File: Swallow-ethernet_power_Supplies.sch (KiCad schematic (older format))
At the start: 31 parts, among them P7 +5V_In, P8 V_In, U12 NCP1529, U13 NCP1529, U14 NCP303LSN09T1G

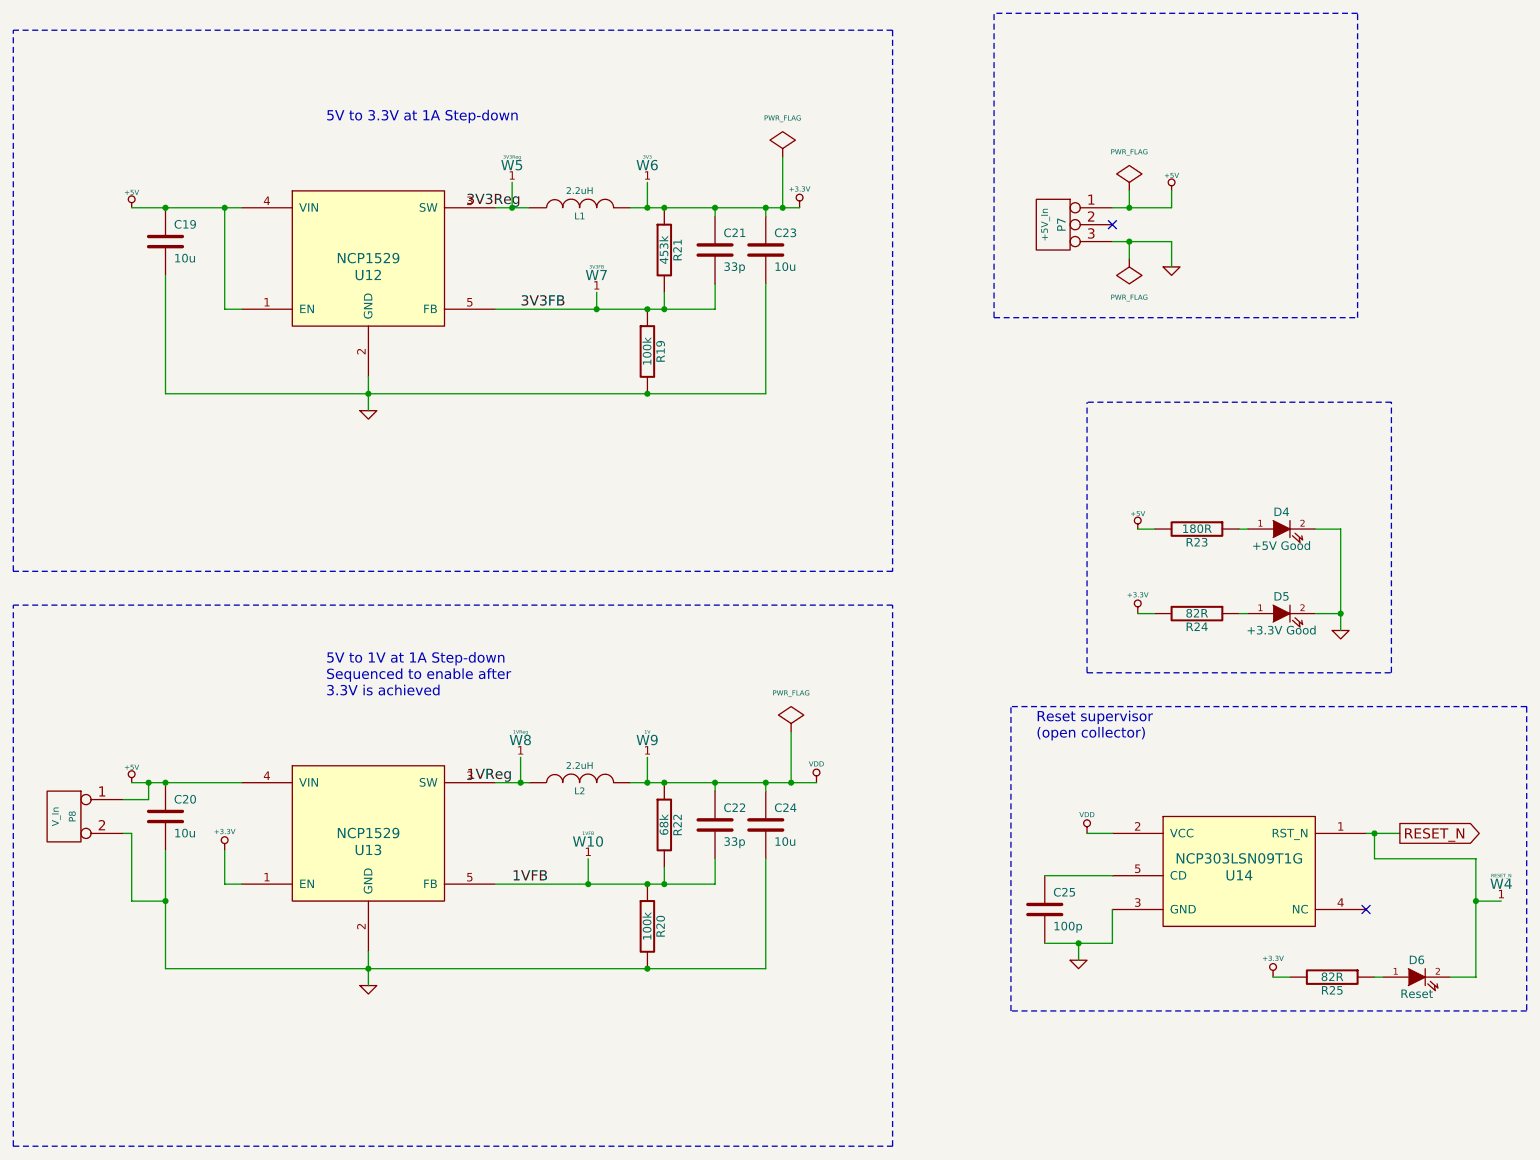
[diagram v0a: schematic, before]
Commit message: Completed schematic.
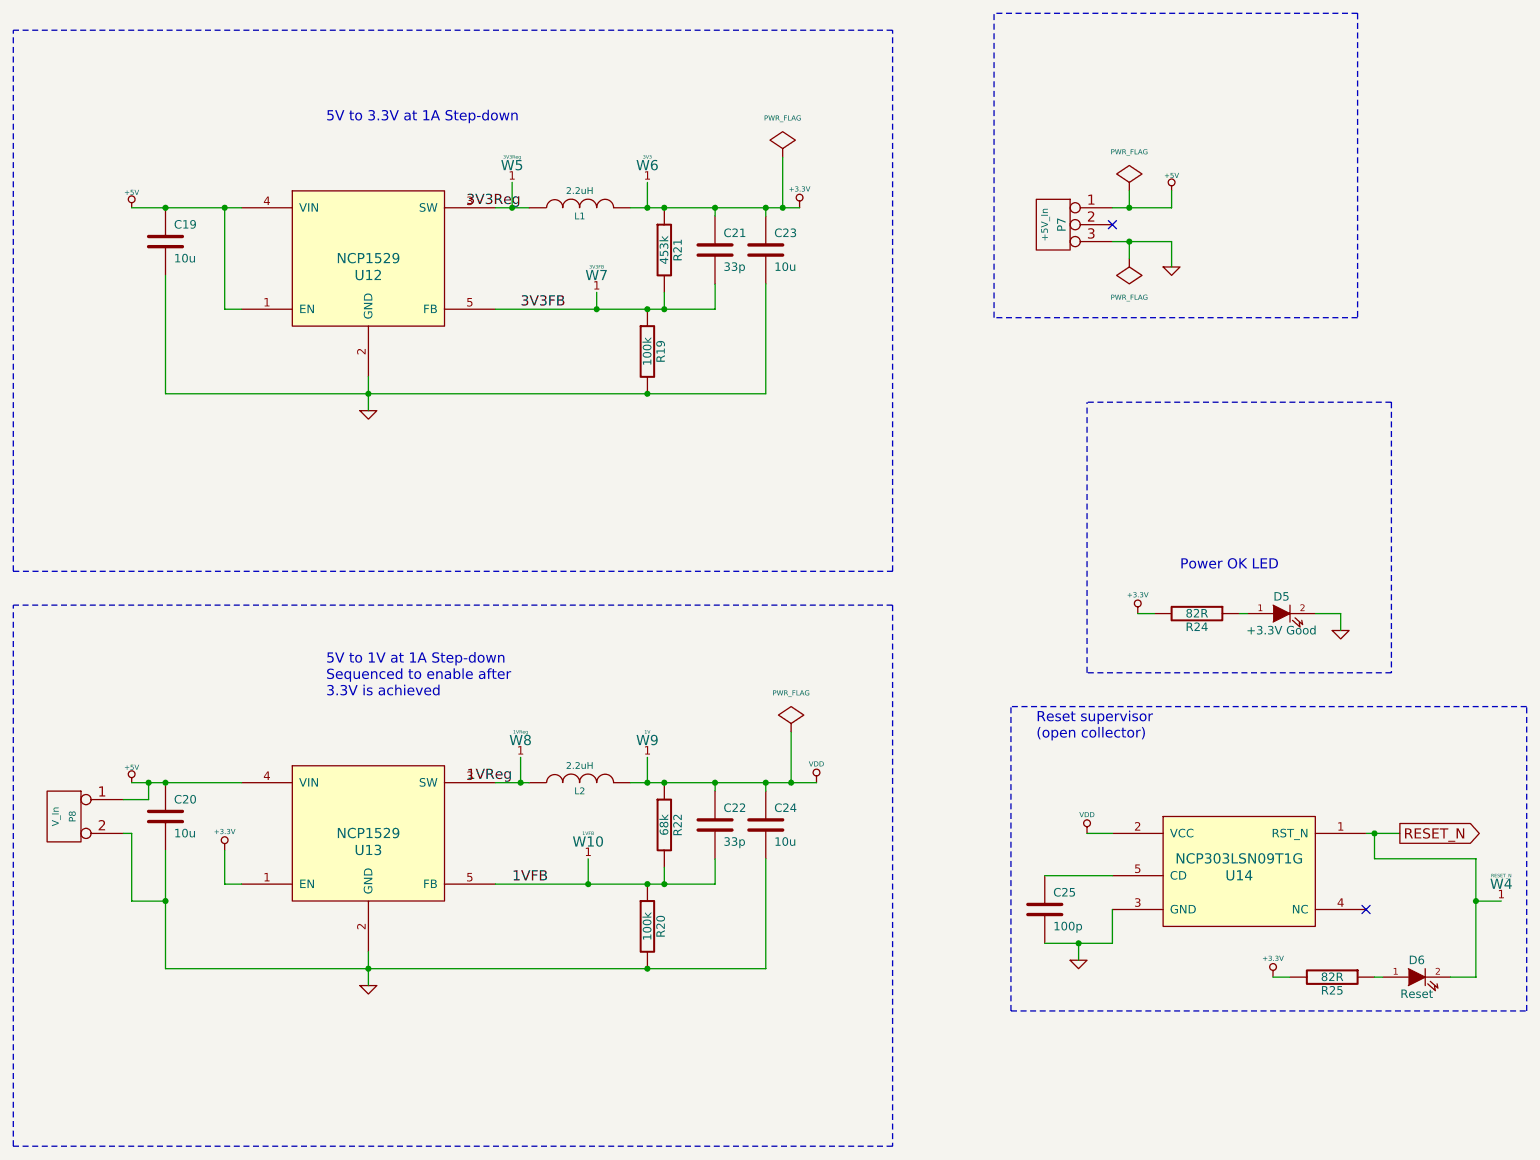
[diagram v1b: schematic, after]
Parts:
- removed D4: +5V Good, X_LED-0603, symbol LED
- removed R23: 180R, SM0402, symbol R
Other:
- note added: "Power OK LED"
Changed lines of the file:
@@
-EESchema Schematic File Version 2  date 30/09/2012 20:10:31
+EESchema Schematic File Version 2  date 30/09/2012 22:11:50
 LIBS:power
 LIBS:device
@@
 Comment4 ""
 $EndDescr
-Wire Wire Line
-	7550 2200 7900 2200
+Text Notes 7950 4150 0    60   ~ 0
+Power OK LED
+Wire Wire Line
+	8900 4500 8900 4400
+Wire Wire Line
+	7650 2200 7650 2300
+Wire Wire Line
+	1700 5700 1750 5700
+Wire Wire Line
+	1750 5700 1750 6100
+Connection ~ 1950 6100
+Wire Wire Line
+	1750 6100 1950 6100
+Connection ~ 4800 5400
+Wire Wire Line
+	4800 5250 4800 5400
+Connection ~ 4000 2000
+Wire Wire Line
+	4000 1850 4000 2000
+Connection ~ 4500 2600
+Wire Wire Line
+	4500 2500 4500 2600
+Connection ~ 9100 5700
+Wire Wire Line
+	9100 5700 9100 5850
+Wire Wire Line
+	9100 5850 9700 5850
+Wire Wire Line
+	9700 5850 9700 6550
+Wire Notes Line
+	6950 6750 6950 4950
+Wire Notes Line
+	6950 6750 10000 6750
+Wire Notes Line
+	10000 6750 10000 4950
+Wire Notes Line
+	10000 4950 6950 4950
+Wire Wire Line
+	9050 5700 9250 5700
+Connection ~ 7350 6350
+Wire Wire Line
+	7350 6450 7350 6350
+Wire Wire Line
+	7150 6350 7550 6350
+Wire Wire Line
+	7550 6350 7550 6150
+Wire Wire Line
+	2400 6000 2300 6000
+Wire Notes Line
+	9200 3150 7400 3150
+Wire Notes Line
+	9200 3150 9200 4750
+Wire Notes Line
+	9200 4750 7400 4750
+Wire Notes Line
+	7400 4750 7400 3150
+Wire Wire Line
+	7700 4400 7800 4400
+Connection ~ 5650 5400
+Wire Wire Line
+	5650 5100 5650 5400
+Wire Wire Line
+	7650 2000 7650 1900
+Connection ~ 7650 2000
+Wire Wire Line
+	7900 2350 7900 2200
+Wire Wire Line
+	5800 5400 4700 5400
+Connection ~ 1950 2000
+Wire Wire Line
+	1750 2000 2400 2000
+Connection ~ 4800 3100
+Wire Wire Line
+	5500 2450 5500 3100
+Wire Wire Line
+	5500 3100 1950 3100
+Connection ~ 4900 2600
+Wire Wire Line
+	3900 2600 5200 2600
+Wire Wire Line
+	5200 2600 5200 2450
+Connection ~ 4900 2000
+Wire Wire Line
+	5200 2000 5200 2050
+Wire Wire Line
+	3900 2000 4100 2000
+Connection ~ 3150 3100
+Wire Wire Line
+	1950 3100 1950 2400
+Wire Wire Line
+	3150 3200 3150 3000
+Wire Wire Line
+	2400 2600 2300 2600
+Wire Wire Line
+	2300 2600 2300 2000
+Connection ~ 2300 2000
+Wire Wire Line
+	4900 2600 4900 2500
+Connection ~ 4800 2600
+Wire Wire Line
+	5500 2050 5500 2000
+Connection ~ 5200 2000
+Wire Wire Line
+	5700 2000 4700 2000
+Connection ~ 5500 2000
+Wire Notes Line
+	1050 4150 1050 950
+Wire Notes Line
+	1050 4150 6250 4150
+Wire Notes Line
+	6250 4150 6250 950
+Wire Notes Line
+	6250 950  1050 950
+Wire Notes Line
+	6250 4350 1050 4350
+Wire Notes Line
+	6250 4350 6250 7550
+Wire Notes Line
+	6250 7550 1050 7550
+Wire Notes Line
+	1050 7550 1050 4350
+Connection ~ 5500 5400
+Connection ~ 5200 5400
+Wire Wire Line
+	5500 5400 5500 5450
+Connection ~ 4800 6000
+Wire Wire Line
+	4900 5900 4900 6000
+Wire Wire Line
+	3150 6600 3150 6400
+Wire Wire Line
+	1950 5800 1950 6500
+Connection ~ 3150 6500
+Wire Wire Line
+	3900 5400 4100 5400
+Wire Wire Line
+	5200 5400 5200 5450
+Connection ~ 4900 5400
+Wire Wire Line
+	5200 5850 5200 6000
+Wire Wire Line
+	5200 6000 3900 6000
+Connection ~ 4900 6000
+Wire Wire Line
+	1950 6500 5500 6500
+Wire Wire Line
+	5500 6500 5500 5850
+Connection ~ 4800 6500
+Wire Wire Line
+	1750 5400 2400 5400
+Connection ~ 1950 5400
+Wire Wire Line
+	7900 1900 7900 2000
+Wire Notes Line
+	9000 850  6850 850
+Wire Notes Line
+	9000 850  9000 2650
+Wire Notes Line
+	9000 2650 6850 2650
+Wire Notes Line
+	6850 2650 6850 850
+Connection ~ 7650 2200
+Wire Wire Line
+	5600 1700 5600 2000
+Connection ~ 5600 2000
+Wire Wire Line
+	8900 4400 8750 4400
+Wire Wire Line
+	8300 4400 8350 4400
+Wire Wire Line
+	7550 5950 7150 5950
+Wire Wire Line
+	7400 5700 7550 5700
+Wire Wire Line
+	9100 6550 9150 6550
+Wire Wire Line
+	9700 6550 9550 6550
+Wire Wire Line
+	8500 6550 8600 6550
+Wire Wire Line
+	9850 6100 9700 6100
+Connection ~ 9700 6100
+Wire Wire Line
+	7900 2000 7550 2000
+Wire Wire Line
+	2300 6000 2300 5800
+Wire Wire Line
+	4800 1850 4800 2000
+Connection ~ 4800 2000
+Wire Wire Line
+	4450 5850 4450 6000
+Connection ~ 4450 6000
+Wire Wire Line
+	4050 5250 4050 5400
+Connection ~ 4050 5400
+Wire Wire Line
+	1700 5500 1850 5500
+Wire Wire Line
+	1850 5500 1850 5400
 Connection ~ 1850 5400
 Wire Wire Line
-	1850 5400 1850 5500
-Wire Wire Line
-	1850 5500 1700 5500
-Connection ~ 4050 5400
-Wire Wire Line
-	4050 5250 4050 5400
-Connection ~ 4450 6000
-Wire Wire Line
-	4450 5850 4450 6000
-Connection ~ 4800 2000
-Wire Wire Line
-	4800 1850 4800 2000
-Wire Wire Line
-	2300 5800 2300 6000
-Wire Wire Line
-	7550 2000 7900 2000
-Connection ~ 9700 6100
-Wire Wire Line
-	9850 6100 9700 6100
-Wire Wire Line
-	8500 6550 8600 6550
-Wire Wire Line
-	9550 6550 9700 6550
-Wire Wire Line
-	9100 6550 9150 6550
-Wire Wire Line
-	7400 5700 7550 5700
-Wire Wire Line
-	7550 5950 7150 5950
-Wire Wire Line
-	8300 4400 8350 4400
-Wire Wire Line
-	7700 3900 7800 3900
-Wire Wire Line
-	8900 4400 8750 4400
-Connection ~ 5600 2000
-Wire Wire Line
-	5600 1700 5600 2000
-Connection ~ 7650 2200
-Wire Notes Line
-	6850 2650 6850 850
-Wire Notes Line
-	6850 2650 9000 2650
-Wire Notes Line
-	9000 2650 9000 850
-Wire Notes Line
-	9000 850  6850 850
-Wire Wire Line
-	7900 2000 7900 1900
-Connection ~ 1950 5400
-Wire Wire Line
-	1750 5400 2400 5400
-Connection ~ 4800 6500
-Wire Wire Line
-	5500 5850 5500 6500
-Wire Wire Line
-	5500 6500 1950 6500
-Connection ~ 4900 6000
-Wire Wire Line
-	3900 6000 5200 6000
-Wire Wire Line
-	5200 6000 5200 5850
-Connection ~ 4900 5400
-Wire Wire Line
-	5200 5400 5200 5450
-Wire Wire Line
-	3900 5400 4100 5400
-Connection ~ 3150 6500
-Wire Wire Line
-	1950 6500 1950 5800
-Wire Wire Line
-	3150 6600 3150 6400
-Wire Wire Line
-	4900 5900 4900 6000
-Connection ~ 4800 6000
-Wire Wire Line
-	5500 5400 5500 5450
-Connection ~ 5200 5400
-Connection ~ 5500 5400
-Wire Notes Line
-	1050 7550 1050 4350
-Wire Notes Line
-	1050 7550 6250 7550
-Wire Notes Line
-	6250 7550 6250 4350
-Wire Notes Line
-	6250 4350 1050 4350
-Wire Notes Line
-	6250 950  1050 950
-Wire Notes Line
-	6250 950  6250 4150
-Wire Notes Line
-	6250 4150 1050 4150
-Wire Notes Line
-	1050 4150 1050 950
-Connection ~ 5500 2000
-Wire Wire Line
-	5700 2000 4700 2000
-Connection ~ 5200 2000
-Wire Wire Line
-	5500 2050 5500 2000
-Connection ~ 4800 2600
-Wire Wire Line
-	4900 2600 4900 2500
-Connection ~ 2300 2000
-Wire Wire Line
-	2300 2000 2300 2600
-Wire Wire Line
-	2300 2600 2400 2600
-Wire Wire Line
-	3150 3200 3150 3000
-Wire Wire Line
-	1950 2400 1950 3100
-Connection ~ 3150 3100
-Wire Wire Line
-	3900 2000 4100 2000
-Wire Wire Line
-	5200 2000 5200 2050
-Connection ~ 4900 2000
-Wire Wire Line
-	5200 2450 5200 2600
-Wire Wire Line
-	5200 2600 3900 2600
-Connection ~ 4900 2600
-Wire Wire Line
-	1950 3100 5500 3100
-Wire Wire Line
-	5500 3100 5500 2450
-Connection ~ 4800 3100
-Wire Wire Line
-	1750 2000 2400 2000
-Connection ~ 1950 2000
-Wire Wire Line
-	5800 5400 4700 5400
-Wire Wire Line
-	7900 2200 7900 2350
-Connection ~ 7650 2000
-Wire Wire Line
-	7650 2000 7650 1900
-Wire Wire Line
-	5650 5100 5650 5400
-Connection ~ 5650 5400
-Wire Wire Line
-	8900 4500 8900 3900
-Wire Wire Line
-	8900 3900 8750 3900
-Connection ~ 8900 4400
-Wire Wire Line
-	7700 4400 7800 4400
-Wire Wire Line
-	8350 3900 8300 3900
-Wire Notes Line
-	7400 4750 7400 3150
-Wire Notes Line
-	7400 4750 9200 4750
-Wire Notes Line
-	9200 4750 9200 3150
-Wire Notes Line
-	9200 3150 7400 3150
-Wire Wire Line
-	2300 6000 2400 6000
-Wire Wire Line
-	7550 6150 7550 6350
-Wire Wire Line
-	7550 6350 7150 6350
-Wire Wire Line
-	7350 6450 7350 6350
-Connection ~ 7350 6350
-Wire Wire Line
-	9050 5700 9250 5700
-Wire Notes Line
-	10000 4950 6950 4950
-Wire Notes Line
-	10000 4950 10000 6750
-Wire Notes Line
-	10000 6750 6950 6750
-Wire Notes Line
-	6950 6750 6950 4950
-Wire Wire Line
-	9700 6550 9700 5850
-Wire Wire Line
-	9700 5850 9100 5850
-Wire Wire Line
-	9100 5850 9100 5700
-Connection ~ 9100 5700
-Wire Wire Line
-	4500 2500 4500 2600
-Connection ~ 4500 2600
-Wire Wire Line
-	4000 1850 4000 2000
-Connection ~ 4000 2000
-Wire Wire Line
-	4800 5250 4800 5400
-Connection ~ 4800 5400
-Wire Wire Line
-	1950 6100 1750 6100
-Connection ~ 1950 6100
-Wire Wire Line
-	1750 6100 1750 5700
-Wire Wire Line
-	1750 5700 1700 5700
-Wire Wire Line
-	7650 2200 7650 2300
+	7900 2200 7550 2200
 NoConn ~ 7550 2100
 $Comp
@@
 $EndComp
 $Comp
-L +5V #PWR092
-U 1 1 4ED17431
-P 7700 3900
-F 0 "#PWR092" H 7700 3990 20  0001 C CNN
-F 1 "+5V" H 7700 3990 30  0000 C CNN
-	1    7700 3900
-	1    0    0    -1
-$EndComp
-$Comp
 L LED D5
 U 1 1 4ED17411
@@
 F 2 "X_LED-0603" H 8550 4400 60  0001 C CNN
 	1    8550 4400
-	1    0    0    -1
-$EndComp
-$Comp
-L LED D4
-U 1 1 4ED1740E
-P 8550 3900
-F 0 "D4" H 8550 4000 50  0000 C CNN
-F 1 "+5V Good" H 8550 3800 50  0000 C CNN
-F 2 "X_LED-0603" H 8550 3900 60  0001 C CNN
-	1    8550 3900
 	1    0    0    -1
 $EndComp
@@
 	0    1    1    0
 $EndComp
-$Comp
-L R R23
-U 1 1 4ED173FE
-P 8050 3900
-F 0 "R23" V 8130 3900 50  0000 C CNN
-F 1 "180R" V 8050 3900 50  0000 C CNN
-F 2 "SM0402" H 8050 3900 60  0001 C CNN
-	1    8050 3900
-	0    1    1    0
-$EndComp
